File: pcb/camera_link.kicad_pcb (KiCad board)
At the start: 2 copper layers, 203.8 x 22.2 mm, 19 parts, among them J1 54602-908LF, J2 Conn_01x09_Female, J3 Conn_01x09_Female, Q1 2N2219, U1 LM741

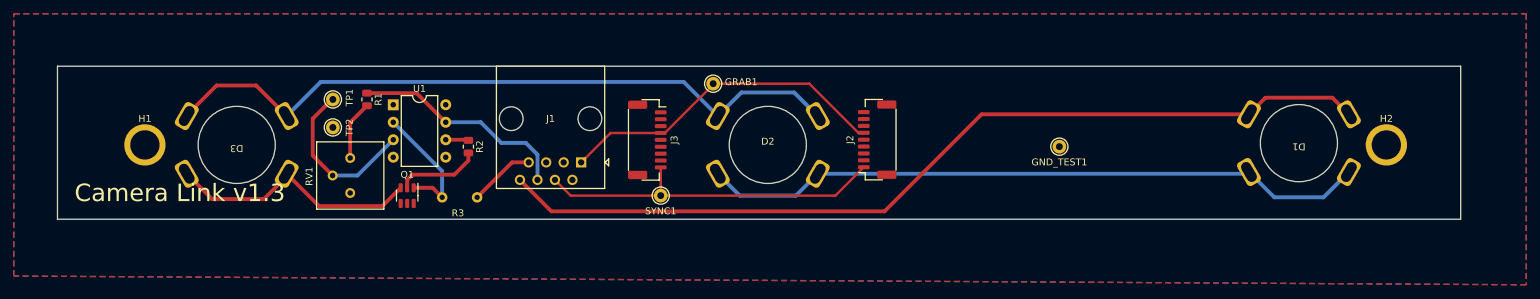
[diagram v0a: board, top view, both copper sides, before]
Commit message: pcb v1.5
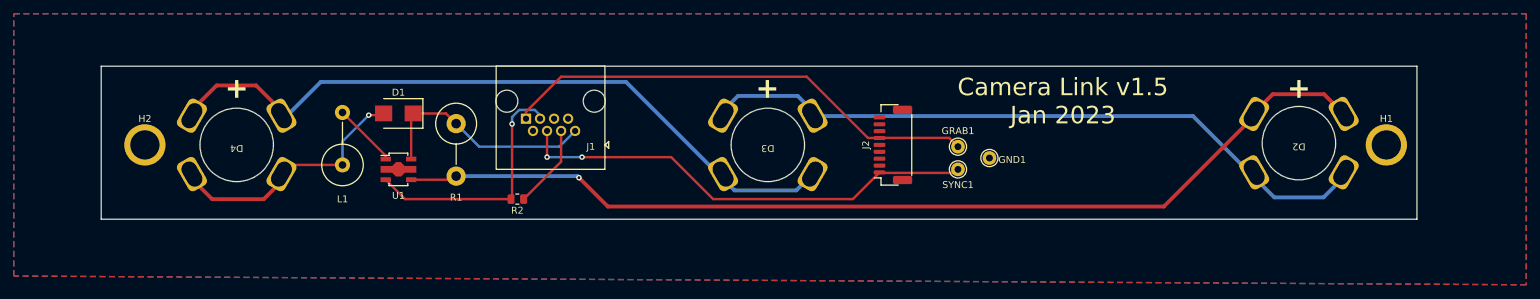
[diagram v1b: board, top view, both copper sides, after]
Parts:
- removed J3: Conn_01x09_Female, asl_footprints:JST_NSH_1x09_VERTICAL
- removed Q1: 2N2219, Package_TO_SOT_SMD:SOT-23-6
- removed the R1 at (91.9, 109.0)
- removed R3: MP915-4.00-1%, asl_footprints:Resistor_power_MP900
- removed RV1: 3386P-1-504TLF, Potentiometer_THT:Potentiometer_Bourns_3386P_Vertical
- removed TP1, TP2: TestPoint, Connector_Pin:Pin_D1.0mm_L10.0mm
- added D1: D, Diode_SMD:D_SMB, F.Cu at (96.5, 111.0)
- added L1: L, Inductor_THT:L_Axial_L14.5mm_D5.8mm_P7.62mm_Vertical_Fastron_HBCC, F.Cu at (88.4, 118.5)
- added R2: R_US, Resistor_SMD:R_0805_2012Metric, F.Cu at (113.8, 123.4)
- J1: value 54602-908LF -> E5J88-00LJG2-L; footprint asl_footprints:RJ45_THP -> asl_footprints:RJ45_THP_tab_on_top
- R1: renamed from R2; value 100 -> R_US; footprint Resistor_SMD:R_0805_2012Metric -> Resistor_THT:R_Axial_DIN0614_L14.3mm_D5.7mm_P7.62mm_Vertical
- U1: value LM741 -> AL8861; footprint Package_DIP:DIP-8_W7.62mm -> Package_TO_SOT_SMD:SOT-89-5
- moved SYNC1 43.3 mm to (177.8, 119.1)
- moved GRAB1 36.7 mm to (177.8, 115.8)
- moved GND1 10.3 mm to (182.4, 117.5)
- moved U1 9.42 mm to (96.5, 119.1)
- moved R1 3.79 mm to (104.9, 112.5)
- moved J1 2.54 mm to (118.6, 109.2)
- moved J2 2.41 mm to (168.4, 115.6)
- turned D3 to 180 degrees
- renumbered D1 to D2, D2 to D3, D3 to D4, GND_TEST1 to GND1, H2 to H1, H1 to H2
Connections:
- D2 pad 2: Net-(D1-A) (its old number) -> Net-(D2-A)
- J1 pad 3: unconnected-(J1-POW-A) -> /LED_CNTRL
- J1 pad 7: /POW_B -> unconnected-(J1-POW-B)
- J1 pad 8: Net-(D1-A) (its old number) -> Net-(D1-K)
- R1 pad 1: Net-(R2-Pad1) -> Net-(D1-K)
- R1 pad 2: Net-(Q1-B) -> Net-(D2-A)
- U1 pad 1: unconnected-(U1-NULL)_1 -> Net-(U1-LX)
- U1 pad 2: Net-(Q1-E) -> GND
- U1 pad 3: Net-(U1-+) -> /LED_CNTRL
- U1 pad 4: GND -> Net-(D2-A)
- U1 pad 5: unconnected-(U1-NULL) -> Net-(D1-K)
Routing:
- net Net-(D2-A): track 0.00 -> 145.8 mm, vias 0 -> 1
- net Net-(D1-A) (its old number): track 130.1 -> 0.00 mm
- net /LED_CNTRL: track 0.00 -> 36.7 mm, vias 0 -> 1
- net Net-(D1-K): track 0.00 -> 33.2 mm
- net Net-(U1-+): track 24.5 -> 0.00 mm
- net /GRAB: track 48.7 -> 70.1 mm
- net Net-(J1-5V): track 32.1 -> 12.2 mm
- net Net-(Q1-E): track 18.6 -> 0.00 mm
- net /SYNC: track 51.6 -> 67.9 mm, vias 0 -> 2
- net Net-(Q1-B): track 12.3 -> 0.00 mm
- net /POW_B: track 9.60 -> 0.00 mm
- net Net-(U1-LX): track 0.00 -> 9.37 mm
- net Net-(R1-Pad2): track 8.61 -> 0.00 mm
- net Net-(D2-K): track 97.5 -> 100.9 mm
- net Net-(R2-Pad1): track 3.33 -> 0.00 mm
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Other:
- board size 203.8 x 22.2 mm -> 191.1 x 22.2 mm
- board text added: "+"
- board text added: "Camera Link v1.5 Jan 2023"
- board text removed: "Camera Link v1.3"
